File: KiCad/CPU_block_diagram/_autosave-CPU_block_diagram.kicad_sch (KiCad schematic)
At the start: 15 parts, among them U1 LM555xM, U2 LM555xM, U3 LM555xM, U4 74LS04, U5 74LS08

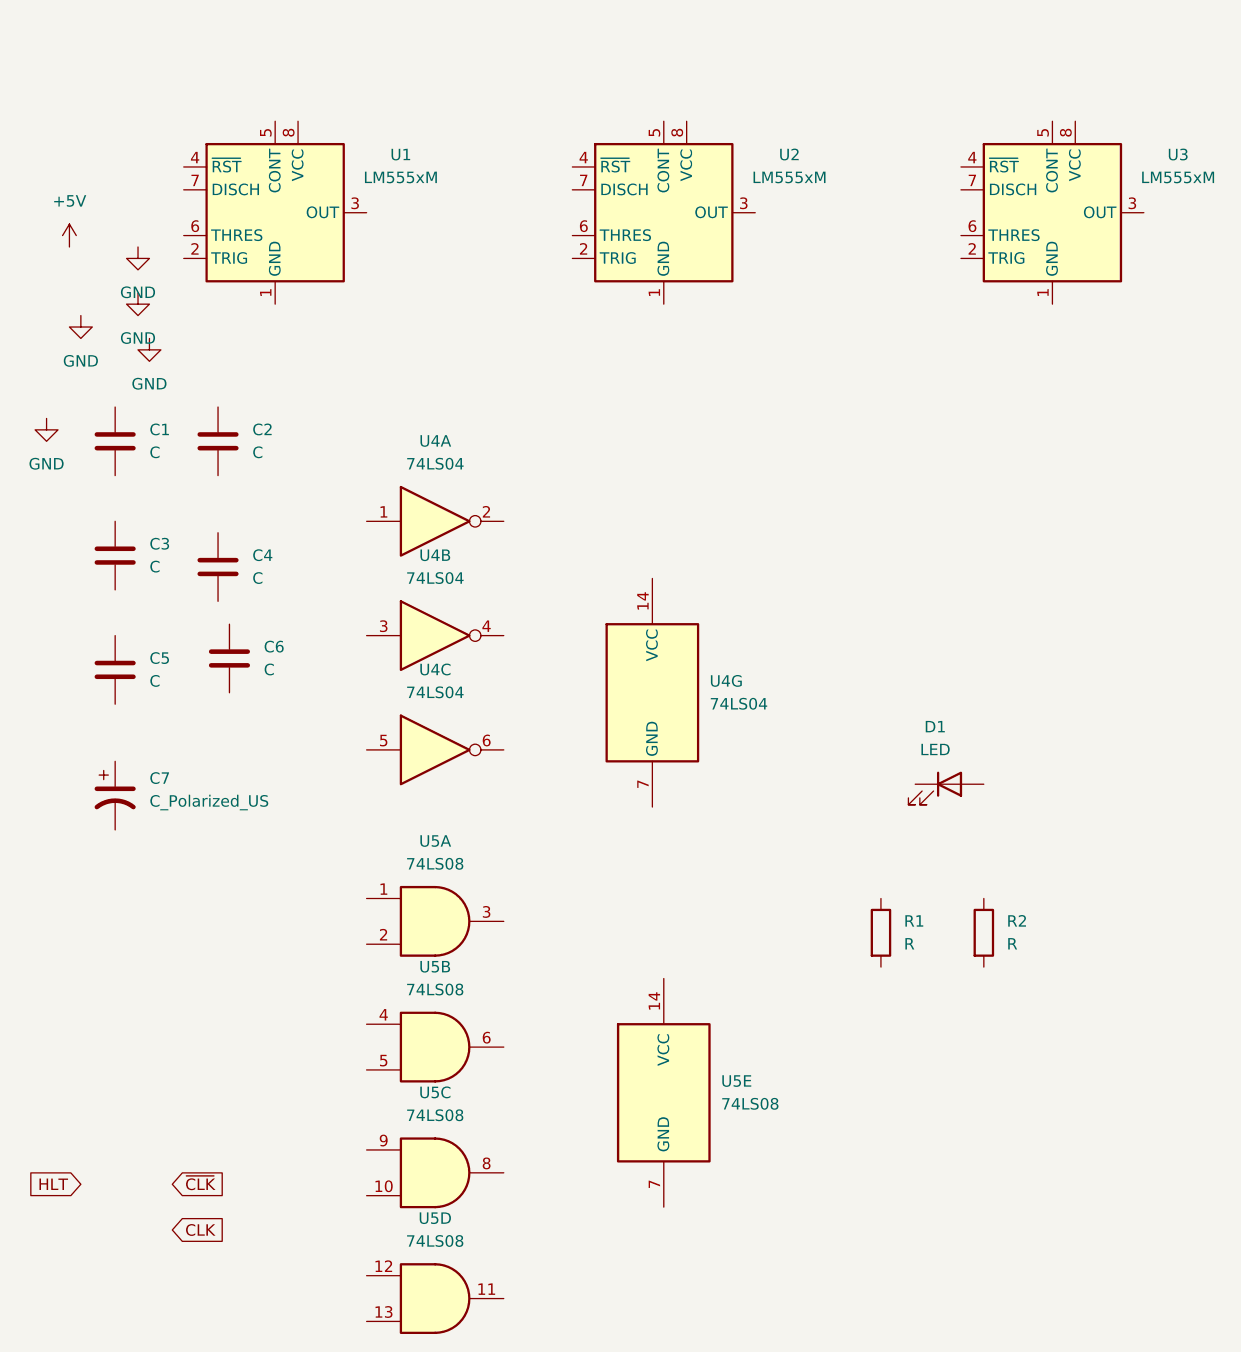
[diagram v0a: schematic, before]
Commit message: vault backup: 2025-12-28 22:43:07
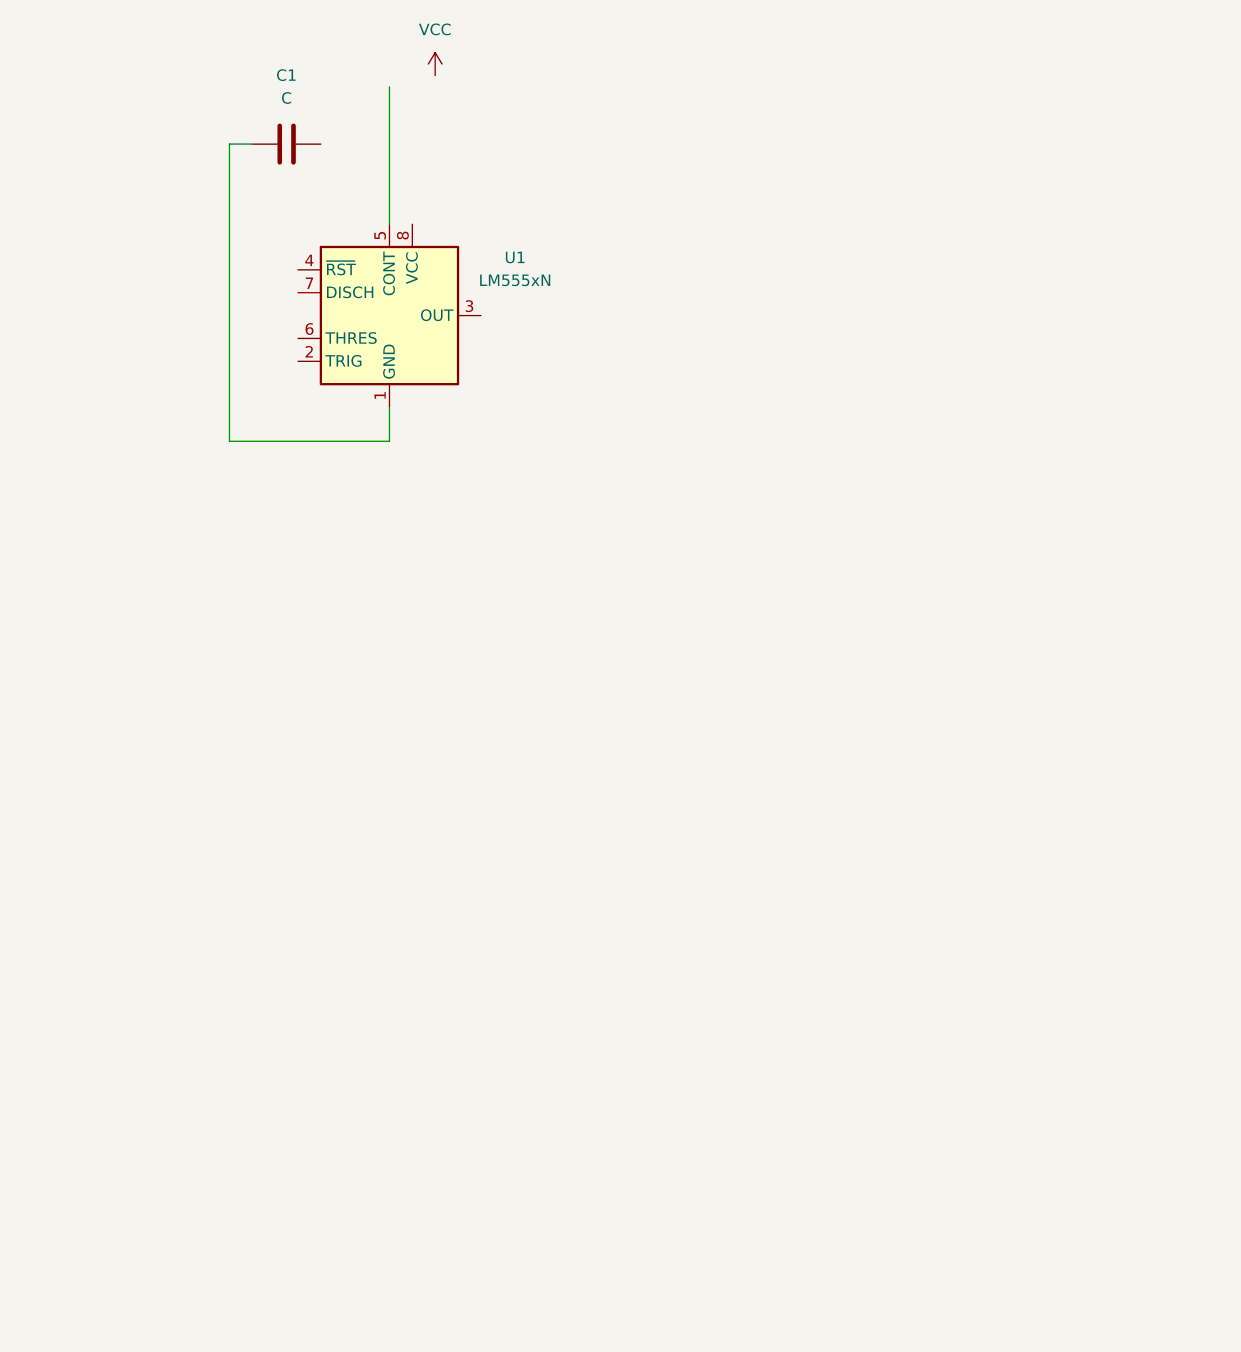
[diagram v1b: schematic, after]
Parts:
- removed C2, C3, C4, C5, C6: C, symbol Device:C
- removed C7: C_Polarized_US, symbol Device:C_Polarized_US
- removed D1: LED, symbol Device:LED
- removed R1, R2: R, symbol Device:R
- removed U1, U2, U3: LM555xM, Package_SO:SOIC-8_3.9x4.9mm_P1.27mm, symbol Timer:LM555xM
- removed U4: 74LS04, symbol 74xx:74LS04
- removed U5: 74LS08, symbol 74xx:74LS08
- added U1: LM555xN, Package_DIP:DIP-8_W7.62mm, symbol Timer:LM555xN
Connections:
- net at C1.1: now also U1.1 (GND)
